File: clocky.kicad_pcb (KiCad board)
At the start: 4 copper layers, 79.9 x 38 mm, 83 parts, among them J1 Bot 50 pin, J2 Bot 40 pin, J3 Top 50 pin, J4 Top 40 pin, J5 Power, J6 JST_PH, J8 Program, U1 HEF4094B, U10 TMP117xxDRV, U2 HEF4094B, U3 HEF4094B, U4 HEF4094B, U5 HEF4094B, U6 HEF4094B, U7 BQ25570, U9 STM32U031C8Ux, Y1 32768Hz

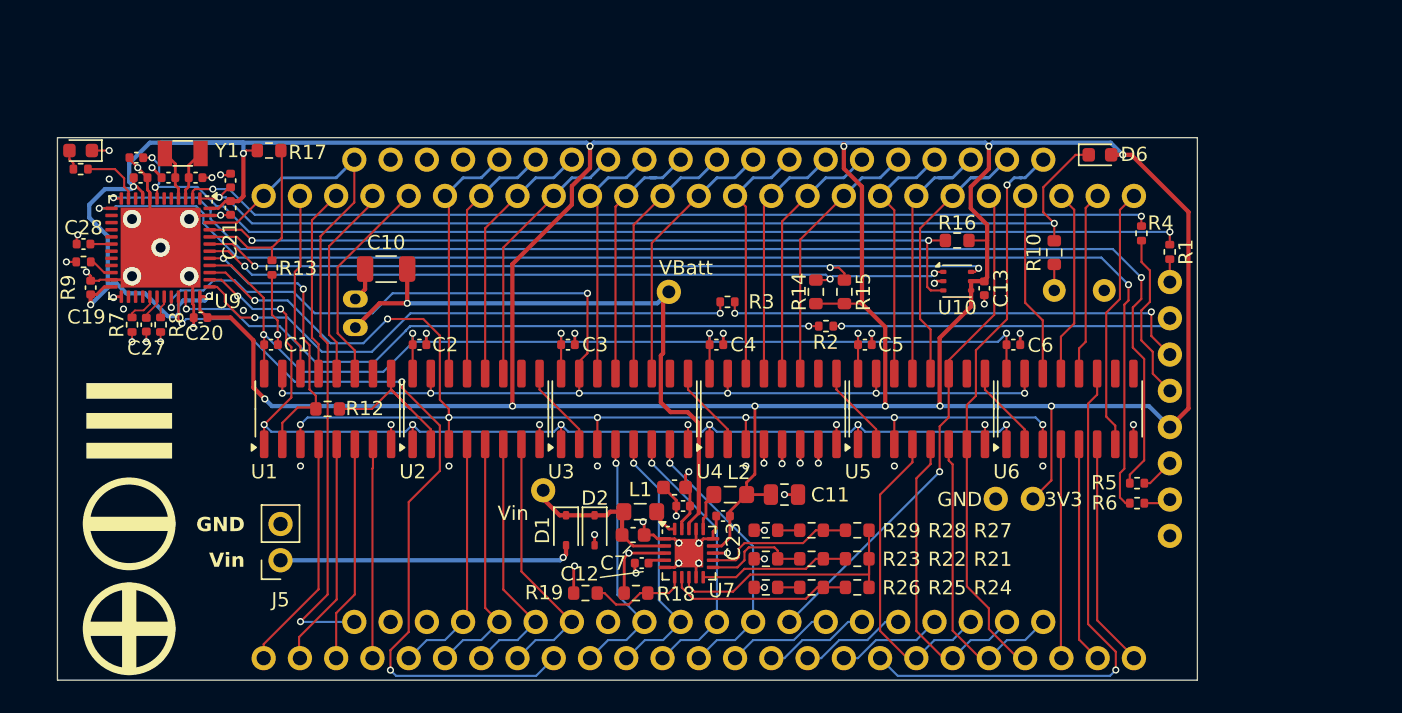
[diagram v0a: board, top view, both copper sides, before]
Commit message: Update PCB layout.  Song and dance with Kicad breaking footprints...
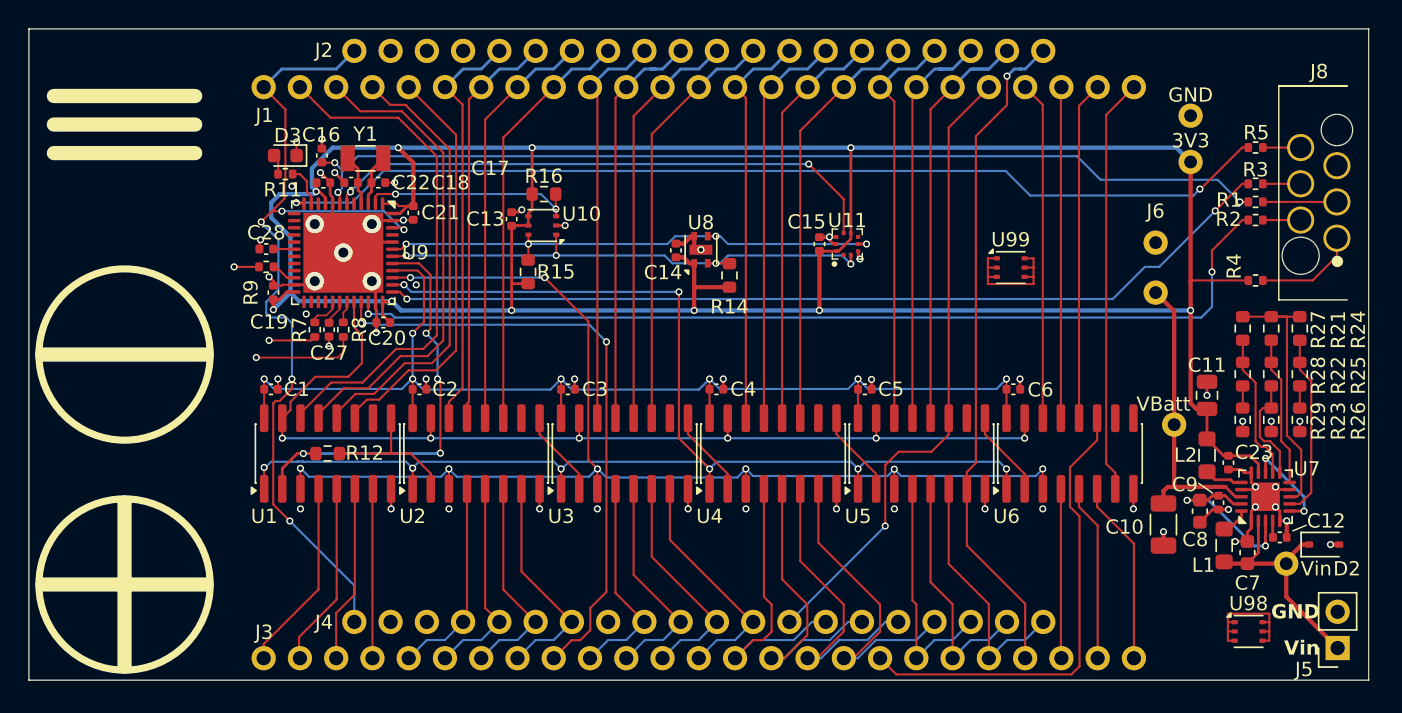
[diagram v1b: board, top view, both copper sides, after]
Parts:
- removed D1: 1N5819WS, Diode_SMD:D_SOD-323
- removed D6: 1N4148, Diode_SMD:D_0603_1608Metric
- removed R10: 100, Resistor_SMD:R_0603_1608Metric
- removed R13: 10k, Resistor_SMD:R_0402_1005Metric
- removed R17: 0, Resistor_SMD:R_0603_1608Metric
- removed R18, R19: 0R, Resistor_SMD:R_0603_1608Metric
- removed R6: 100, Resistor_SMD:R_0402_1005Metric
- added U11: ENS220, Parts:ENS220, F.Cu at (160.4, 88.5)
- added U8: ENS212, Package_DFN_QFN:AMS_QFN-4-1EP_2x2mm_P0.95mm_EP0.7x1.6mm, F.Cu at (150.2, 88.8)
- added U98: TMP117xxDRV, Parts:WSON-6-1EP_2x2mm_P0.65mm_NoEP, F.Cu at (188.5, 115.6)
- added U99: TMP117xxDRV, Parts:WSON-6-1EP_2x2mm_P0.65mm_NoEP, F.Cu at (171.8, 90.1)
- C15: value 1F -> 0u1; footprint Capacitor_THT:C_Radial_D8.0mm_H11.5mm_P3.50mm -> Capacitor_SMD:C_0402_1005Metric; moved to F.Cu
- C16: value 0u1 -> 10n
- J6: value JST_PH -> CAP; footprint Connector_JST:JST_PH_B2B-PH-K_1x02_P2.00mm_Vertical -> Parts:TwoPin_P3.5mm; moved to F.Cu
- J8: value Program -> Skedd; footprint Parts:PinHeader_1x08_P2.54mm_Vertical -> Parts:Skedd6; moved to F.Cu
- R21: value 845k -> 634k
- R22: value 5M6 -> 6M2
- R23: value 3M3 -> 3M9
- R24: value 6M8 -> 5M1
- R25: value 150k -> 330k
- R26: value 2M7 -> 3M9
- U7: footprint Package_DFN_QFN:QFN-20-1EP_3.5x3.5mm_P0.5mm_EP2x2mm -> Parts:QFN-20-1EP_3.5x3.5mm_P0.5mm_EP2x2mm
- U9: footprint Package_DFN_QFN:QFN-48-1EP_7x7mm_P0.5mm_EP5.6x5.6mm -> Parts:QFN-48-1EP_7x7mm_P0.5mm_EP5.6x5.6mm
- moved J5 74.3 mm to (194.8, 116.8)
- moved C10 57.3 mm to (182.6, 108.1), turned to 90 degrees
- moved J6 56.1 mm to (182.0, 90.1), turned to 0 degrees
- moved TP7 52.3 mm to (191.2, 110.8), turned to 90 degrees
- moved D2 51.1 mm to (193.8, 109.5), turned to 0 degrees
- moved C12 44.7 mm to (190.7, 109.0), turned to 0 degrees
- moved C7 43.0 mm to (188.4, 110.1), turned to 90 degrees
- moved L1 41.0 mm to (186.8, 109.6), turned to 90 degrees
- moved U7 40.6 mm to (189.7, 106.2), turned to 90 degrees
- moved R26 39.2 mm to (192.1, 100.8), turned to -90 degrees
- moved C14 38.4 mm to (148.4, 88.9), turned to 90 degrees
- moved R3 37.9 mm to (189.0, 84.2)
- moved C9 37.5 mm to (186.4, 106.6), turned to 90 degrees
- moved R25 37.3 mm to (192.1, 97.6), turned to -90 degrees
- moved C8 36.8 mm to (185.1, 107.2), turned to 90 degrees
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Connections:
- net /Extra renamed /Menu
- net /ExtraCS renamed /MenuC
- net /PTX renamed /dTX
- net /TouchCS renamed /TouchC
- C14 pad 1: /RESET -> +3V3
- C15 pad 1: Net-(C15-Pad1) -> +3V3
- C16 pad 1: /VCap -> /RESET
- J5 pad 1: Net-(D1-A) -> /Vin
- J8 pad 1: /PRST -> /d3V3
- J8 pad 2: /PSWD -> /dSWD
- J8 pad 3: /PSWC -> /dRST
- J8 pad 4: /PRTC -> /dSWC
- J8 pad 5: +3V3 -> GND
- R1 pad 1: /PRST -> /dRST
- R2 pad 1: /PSWD -> /SWDIO
- R2 pad 2: /SWDIO -> /dSWD
- R3 pad 1: /PSWC -> /dSWC
- R4 pad 1: /PRTC -> /d3V3
- R4 pad 2: /RTCOUT -> +3V3
- U7 pad 6: Net-(U7-VOUT_EN) -> /VBatOK
- U9 pad 1: /VCap -> +3V3
- U9 pad 13: /SERRX -> unconnected-(U9-PA3-Pad13)
- U9 pad 2: /RTCOUT -> /Alert
- U9 pad 25: /VBatOK -> unconnected-(U9-PB12-Pad25)
- U9 pad 44: /BOOT0 -> GND
- U9 pad 45: /Alert -> unconnected-(U9-PB8-Pad45)
- U9 pad 6: unconnected-(U9-PF1-Pad6) -> /Press
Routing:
- net /SERRX: track 91.7 -> 0.00 mm, vias 2 -> 0
- net +3V3: track 294.2 -> 218.7 mm, vias 14 -> 10
- net /VCap: track 69.7 -> 0.00 mm, vias 2 -> 0
- net /RTCOUT: track 68.5 -> 0.00 mm, vias 2 -> 0
- net /VBatOK: track 54.7 -> 6.84 mm, vias 3 -> 2
- net /Alert: track 56.4 -> 15.2 mm
- net /Press: track 0.00 -> 39.7 mm, vias 0 -> 2
- net /PSWC: track 33.6 -> 0.00 mm, vias 2 -> 0
- net /OE: track 97.8 -> 72.4 mm, vias 8 -> 6
- net /PSWD: track 23.8 -> 0.00 mm, vias 1 -> 0
- net /SWCLK: track 39.9 -> 63.5 mm
- net /VBatt: track 44.3 -> 20.9 mm, vias 1 -> 0
- net /Q1E: track 12.7 -> 35.9 mm
- net Net-(D1-A): track 20.8 -> 0.00 mm, vias 1 -> 0
- net /SERTX: track 90.6 -> 70.3 mm
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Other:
- board size 79.9 x 38 mm -> 93.9 x 45.6 mm
- board text removed: "3V7"
- board text removed: "RST"
- board text removed: "RTC"
- board text removed: "RX"
- board text removed: "SWC"
- board text removed: "SWD"
- board text removed: "TX"
- board text removed: "≡"
